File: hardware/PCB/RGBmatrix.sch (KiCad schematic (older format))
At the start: 41 parts

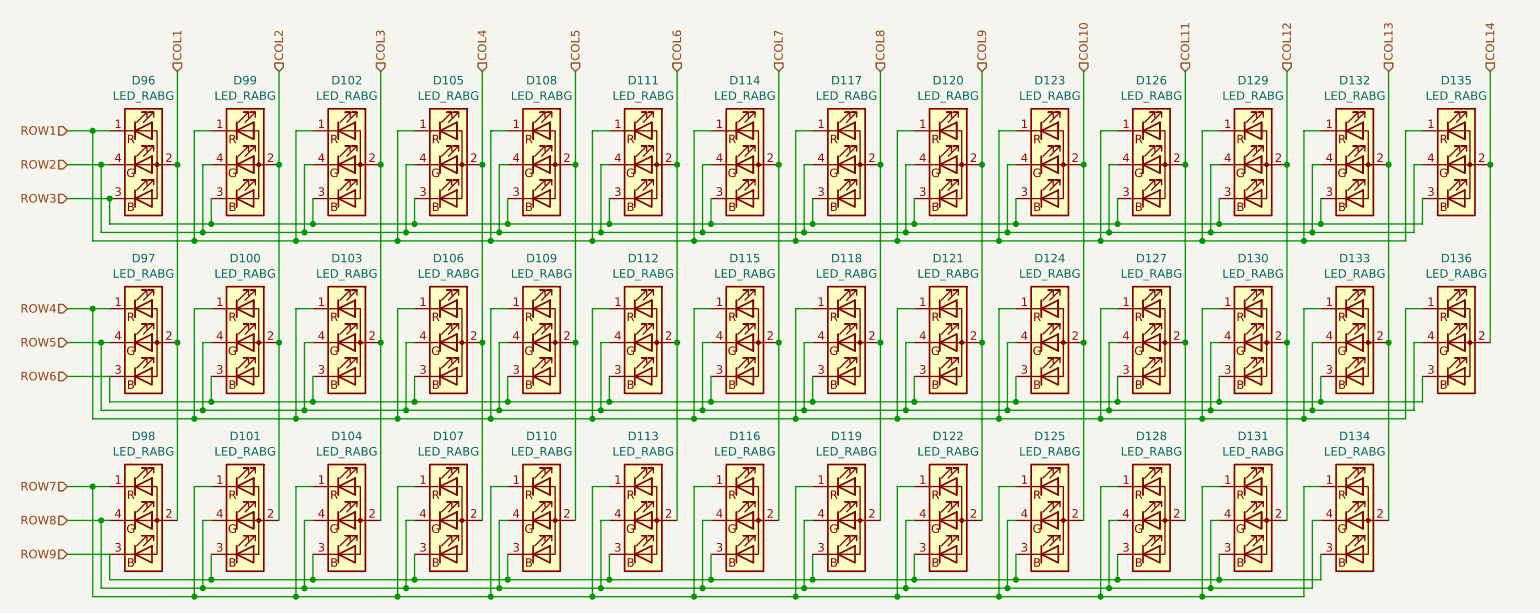
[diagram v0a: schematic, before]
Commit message: making progress
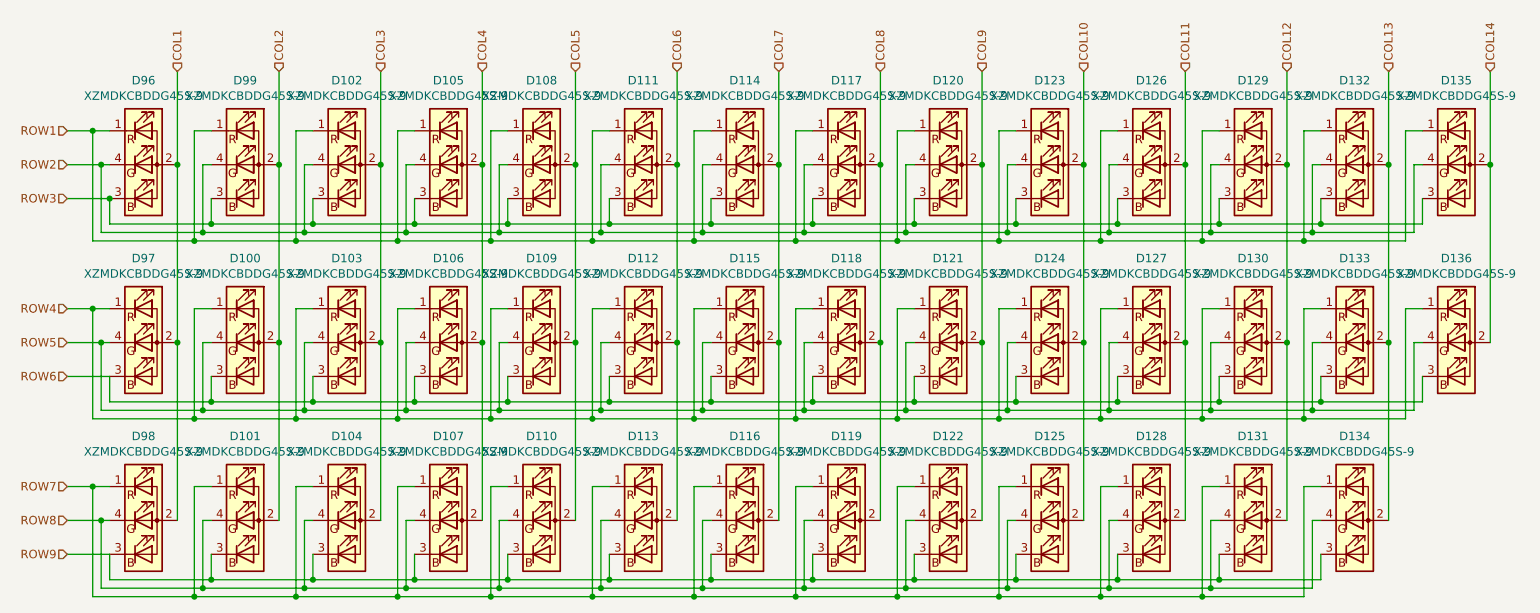
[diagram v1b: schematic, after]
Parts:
- D100, D101, D102, D103, D104, D105, D106, D107, D108, D109, D110, D111, D112, D113, D114, D115, D116, D117, D118, D119, D120, D121, D122, D123, D124, D125, D126, D127, D128, D129, D130, D131, D132, D133, D134, D135, D136, D96, D97, D98, D99: value LED_RABG -> XZMDKCBDDG45S-9
